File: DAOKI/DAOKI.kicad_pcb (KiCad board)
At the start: 2 copper layers, 46 x 19 mm, 16 parts, among them J1 CON1, U1 LG206D, U2 LM393

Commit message: add PCB notes
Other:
- rule trace_min: 0.2 -> 0.5
- rule via_min_size: 0.4 -> 1
- board text added: "Grilla de posicionamiento 1mm Grilla de ruteo 0,5mm Ancho de pista 0,5 mm Diámetro de agujero 0,5 mm Diámetro de pad o vía 1,0 mm Separación entre pistas 0,45 mm Separación entre pista y pad/vía 0,45 mm Separación entre cobre y borde de la placa 0,5 mm Separación entre componentes 0,45 (excepto U1)"
- board text added: "Se uso la información técnica de Mayer SA http://www.mayerpcb.com/informacion-tecnica.html"

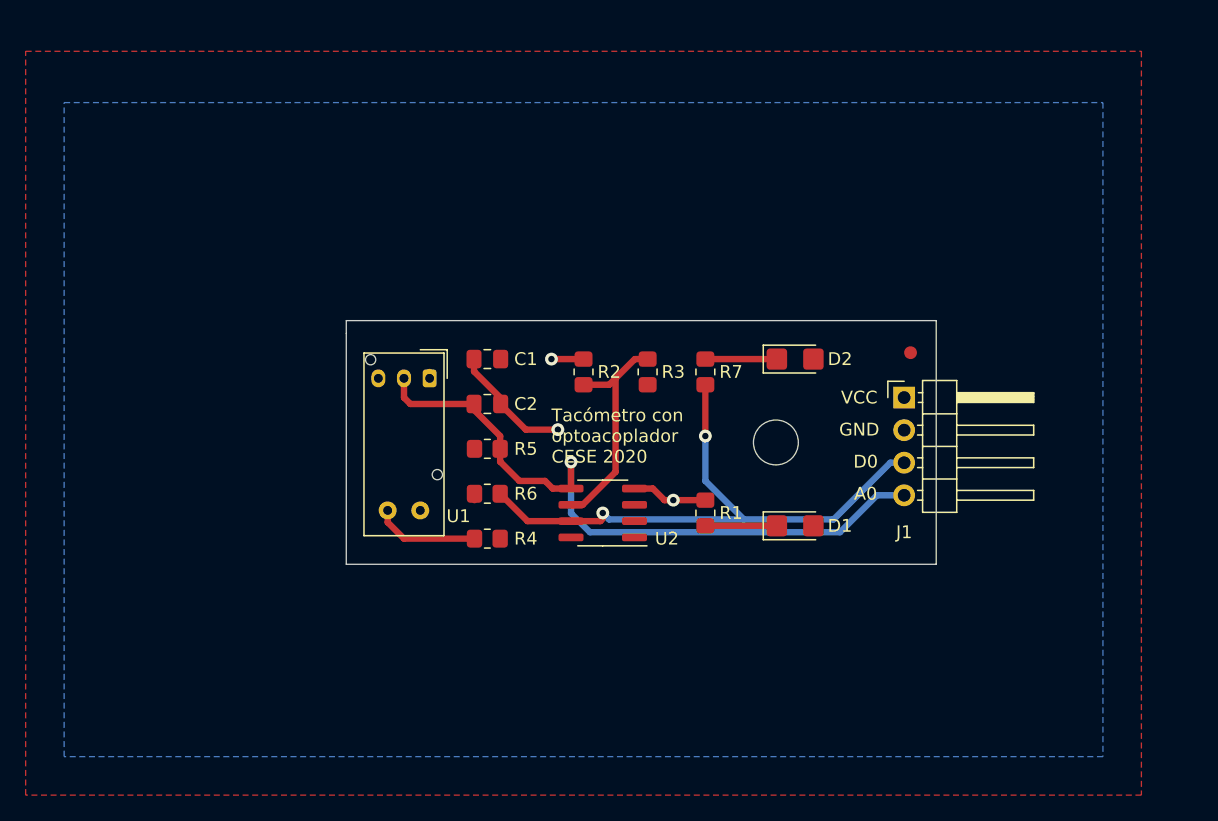
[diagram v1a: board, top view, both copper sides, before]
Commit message: final fixies on notes to PCB maker
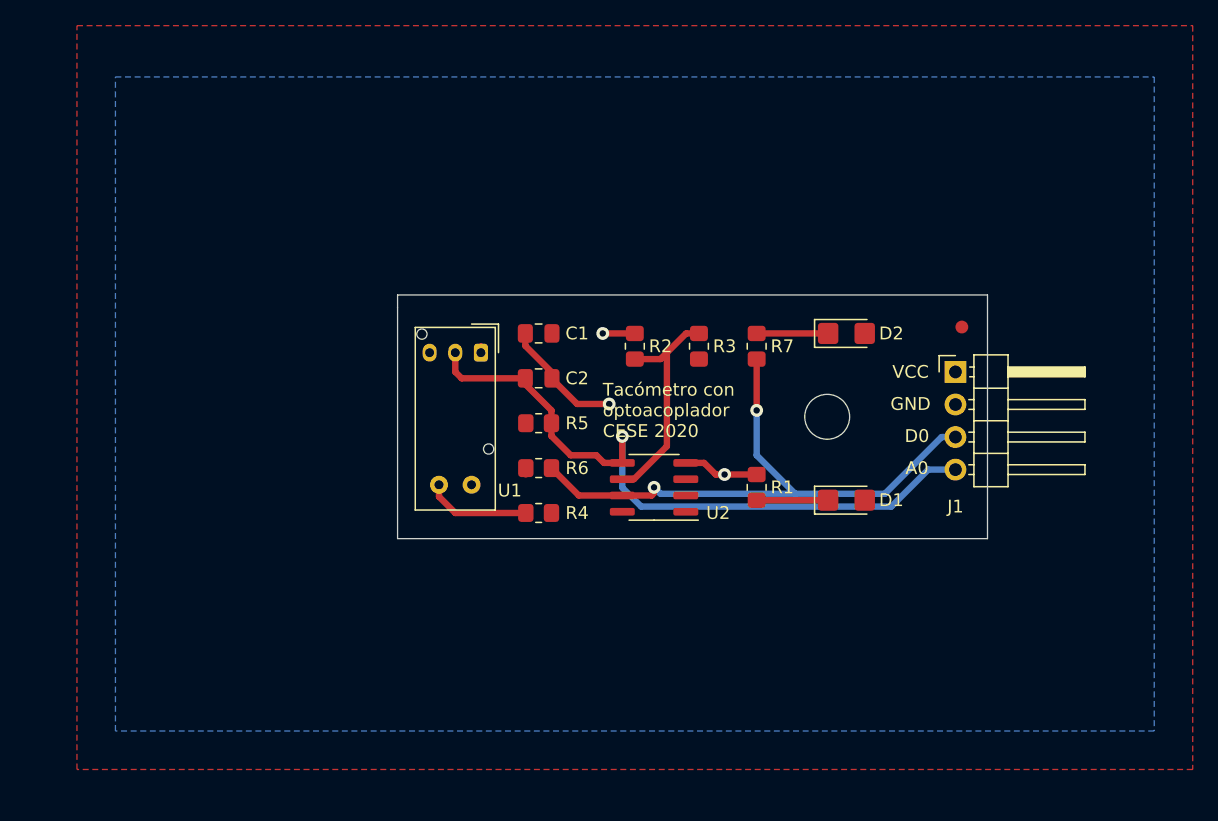
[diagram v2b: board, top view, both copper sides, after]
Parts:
- moved C1 4.47 mm to (143.0, 90.0)
- moved C2 4.47 mm to (143.0, 93.5)
- moved D1 4.47 mm to (167.0, 103.0)
- moved D2 4.47 mm to (167.0, 90.0)
- moved FID1 4.47 mm to (176.0, 89.5)
- moved H1 4.47 mm to (165.5, 96.5)
- moved J1 4.47 mm to (175.5, 93.0)
- moved R1 4.47 mm to (160.0, 102.0)
- moved R2 4.47 mm to (150.5, 91.0)
- moved R3 4.47 mm to (155.5, 91.0)
- moved R4 4.47 mm to (143.0, 104.0)
- moved R5 4.47 mm to (143.0, 97.0)
- moved R6 4.47 mm to (143.0, 100.5)
- moved R7 4.47 mm to (160.0, 91.0)
- moved U1 4.47 mm to (138.5, 91.5)
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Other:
- board text added: "Grilla de posicionamiento 1mm Grilla de ruteo 0,5mm Ancho de pista 0,5 mm Diámetro de agujero 0,5 mm Diámetro de pad o vía 1,0 mm Separación entre pistas 0,45 mm Separación entre pista y pad/vía 0,45 mm Separación entre cobre y borde de la placa 0,5 mm Separación entre componentes 0,45 Recubrimiento de pads: Cu + Flux Terminaciones de Pads: HASL Material PCB: FR4 PCB doble faz"
- board text removed: "Grilla de posicionamiento 1mm Grilla de ruteo 0,5mm Ancho de pista 0,5 mm Diámetro de agujero 0,5 mm Diámetro de pad o vía 1,0 mm Separación entre pistas 0,45 mm Separación entre pista y pad/vía 0,45 mm Separación entre cobre y borde de la placa 0,5 mm Separación entre componentes 0,45 (excepto U1)"
